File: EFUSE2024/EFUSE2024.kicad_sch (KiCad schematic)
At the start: 44 parts, among them Q3 CSD19532Q5B, Q4 CSD19532Q5B, Q7 BSS138, U1 TPS26630RGE, U2 TPS26630RGE, U3 TPS26630RGE, U5 TPS26631PWP, U6 TPS26631PWP, U7 TPS26630RGE

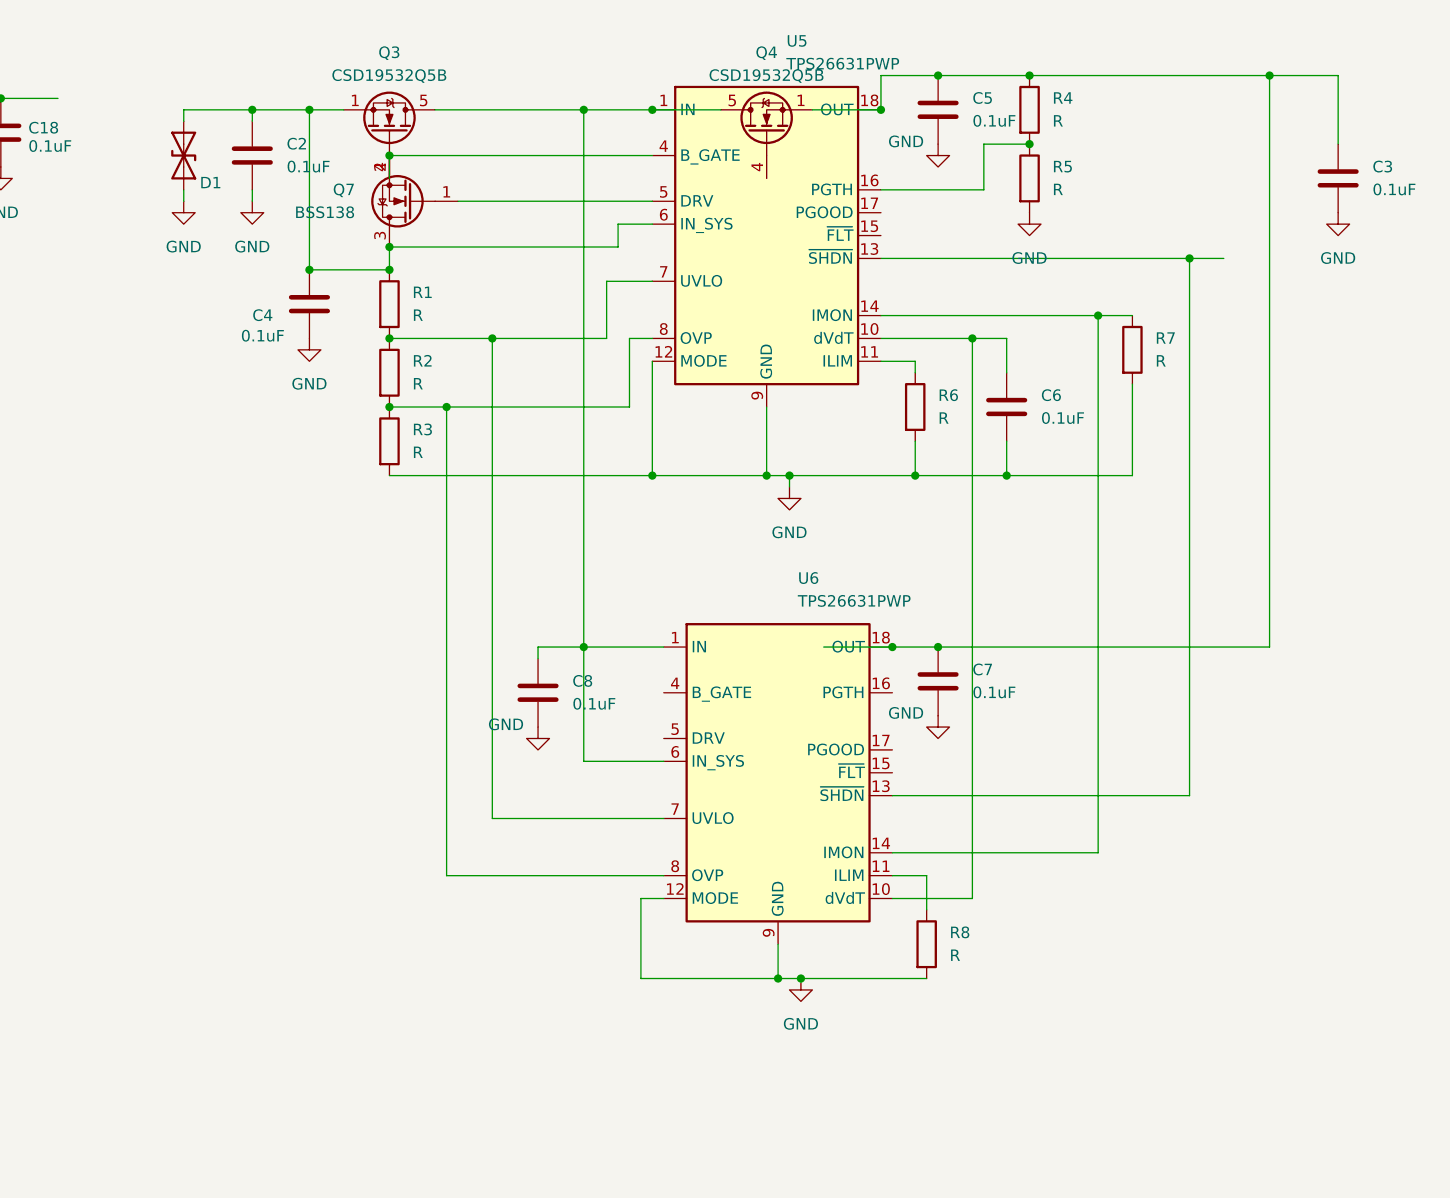
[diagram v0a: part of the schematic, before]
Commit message: deleted two
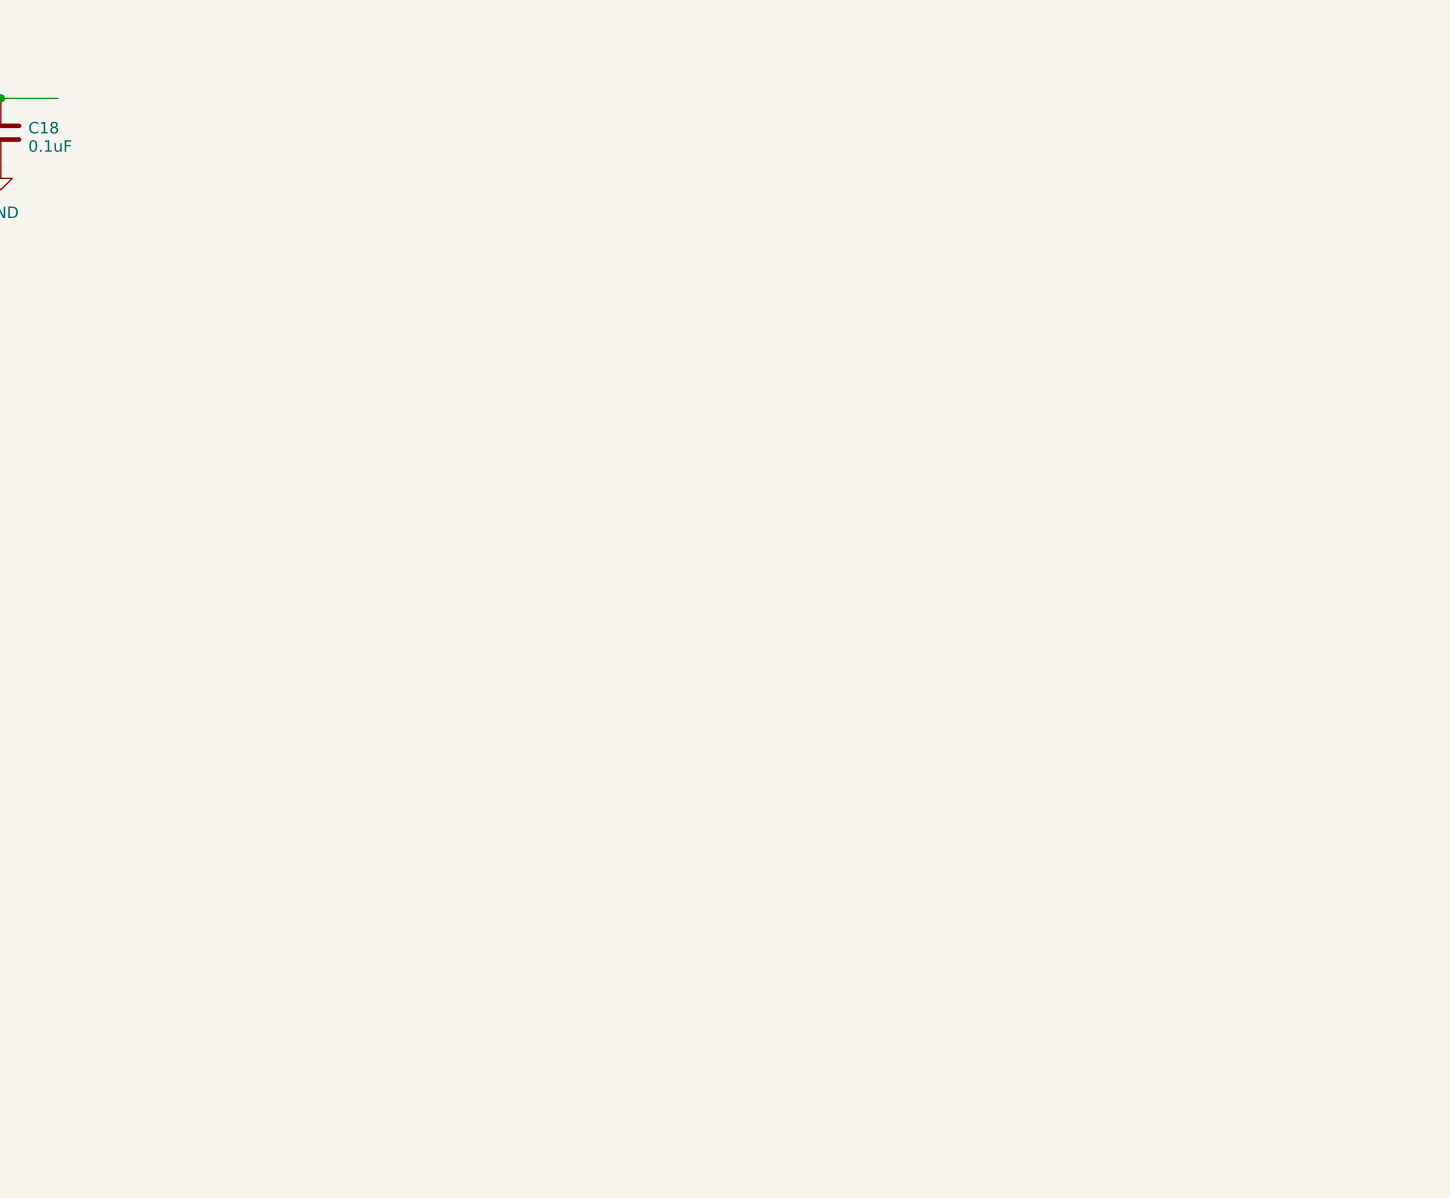
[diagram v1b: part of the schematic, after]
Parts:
- removed C2, C3, C4, C5, C6, C7, C8: 0.1uF, symbol Device:C
- removed D1: 1.5SMCxxCA, Diode_SMD:D_SMC, symbol Diode:1.5SMCxxCA
- removed Q3, Q4: CSD19532Q5B, Package_TO_SOT_SMD:TDSON-8-1, symbol Transistor_FET:CSD19532Q5B
- removed Q7: BSS138, Package_TO_SOT_SMD:SOT-23, symbol Transistor_FET:BSS138
- removed R1, R2, R3, R4, R5, R6, R7, R8: R, symbol Device:R
- removed U5, U6: TPS26631PWP, Package_SO:HTSSOP-20-1EP_4.4x6.5mm_P0.65mm_EP3.4x6.5mm_Mask2.96x2.96mm_ThermalVias, symbol Power_Management:TPS26631PWP
